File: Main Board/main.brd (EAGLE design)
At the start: 76.2 x 37.6 mm, 7 parts

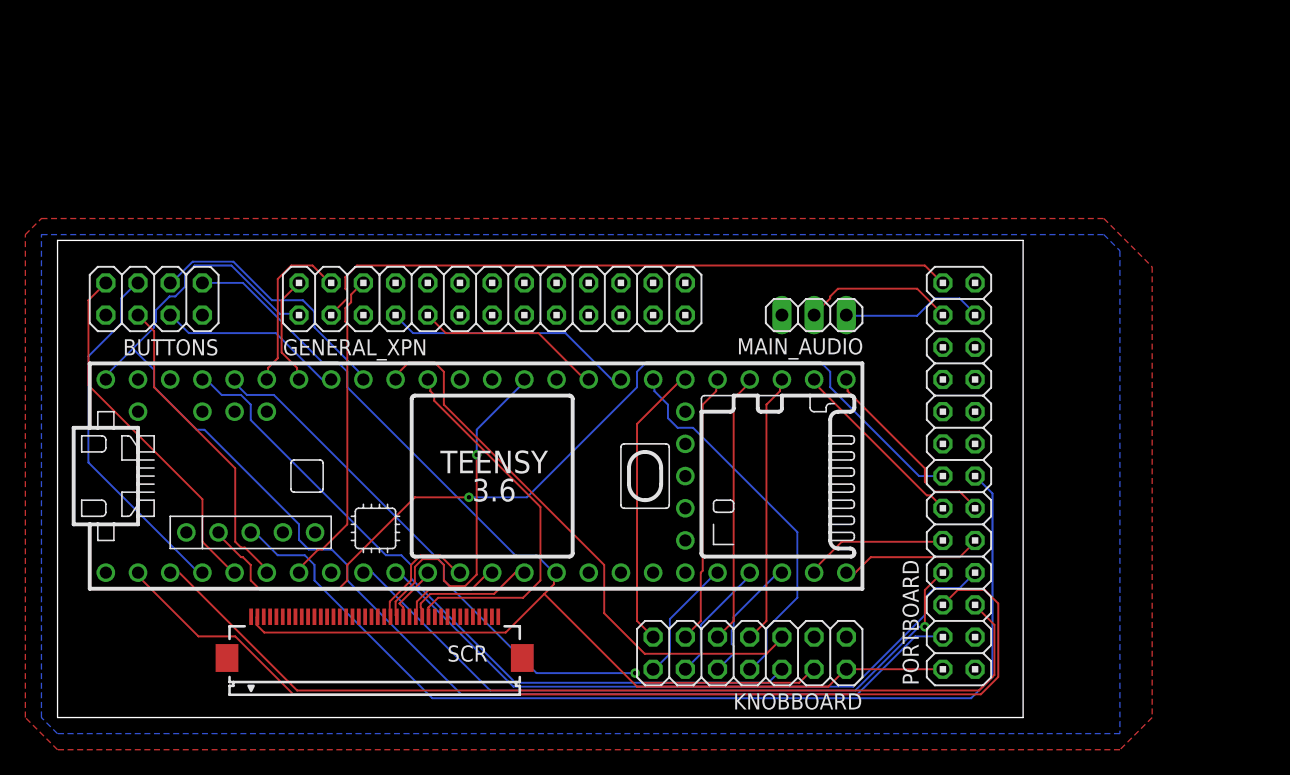
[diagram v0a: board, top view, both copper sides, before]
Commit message: Main Board Complete!
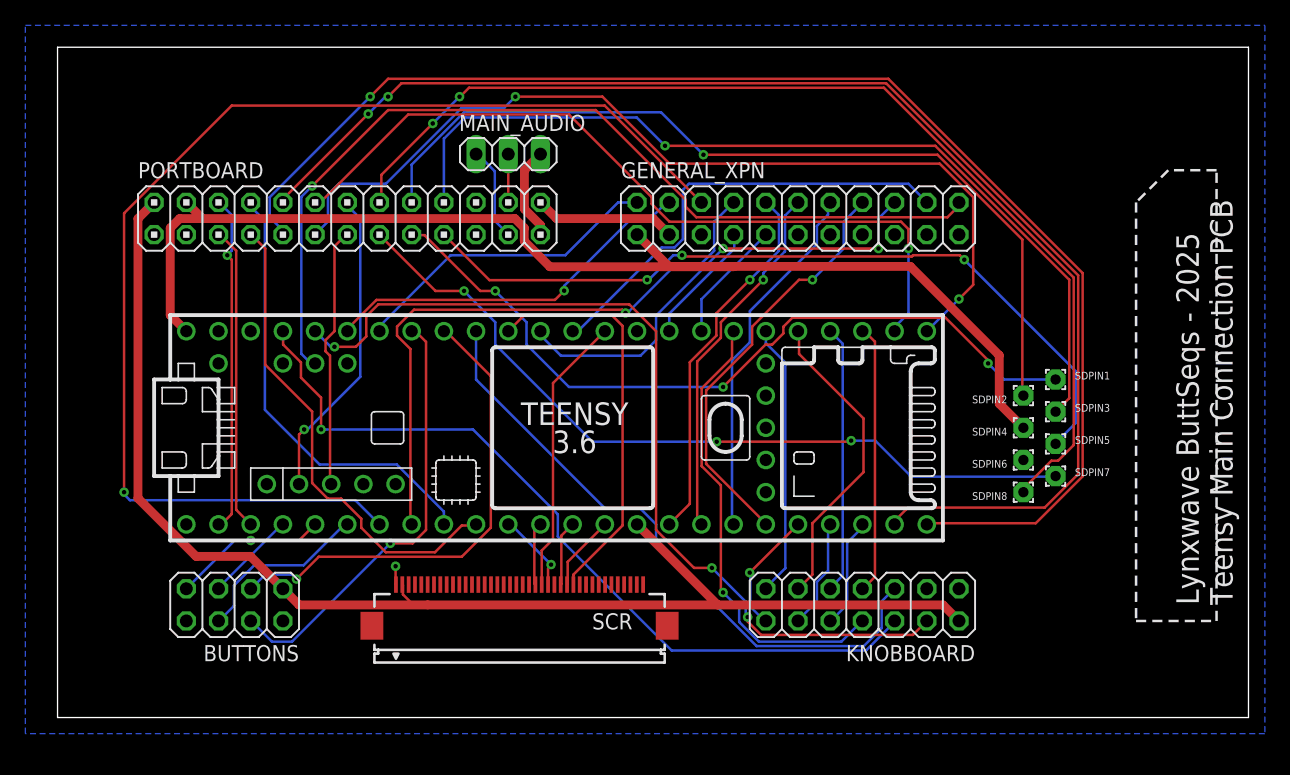
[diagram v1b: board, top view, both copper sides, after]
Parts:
- added SDPIN1, SDPIN2, SDPIN3, SDPIN4, SDPIN5, SDPIN6, SDPIN7, SDPIN8: (no value), wirepad:1,6/0,8
- GENERAL_XPN: device pinhead:2X13 -> pinhead:2X11
- moved PORTBOARD 52.4 mm to (22.9, 39.4), turned to 0 degrees
- moved MAIN_AUDIO 27.3 mm to (35.6, 44.5), turned to 0 degrees
- moved BUTTONS 25.0 mm to (14.0, 8.89)
- moved GENERAL_XPN 25.0 mm to (58.4, 39.4)
- moved SCR 11.7 mm to (36.4, 7.24)
- moved KNOBBOARD 9.67 mm to (63.5, 8.89)
- moved TEENSY_3.6 7.41 mm to (38.1, 22.9)
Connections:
- net AUDIO_L renamed OUTPUT_L
- net AUDIO_R renamed OUTPUT_R
- net SPI_CLK renamed XPN_CLK
- net SPI_MISO renamed XPN_MISO
- net SPI_MOSI renamed XPN_MOSI
- removed net AUDIO_0: GENERAL_XPN.11
- removed net AUDIO_1: GENERAL_XPN.13
- removed net AUDIO_2: GENERAL_XPN.15
- removed net AUDIO_3: GENERAL_XPN.17
- removed net AUDIO_4: GENERAL_XPN.19
- removed net AUDIO_5: GENERAL_XPN.21
- removed net AUDIO_6: GENERAL_XPN.23
- removed net AUDIO_7: GENERAL_XPN.25
- removed net N$10: TEENSY_3.6.25
- removed net N$11: TEENSY_3.6.26
- removed net N$12: TEENSY_3.6.27
- removed net N$25: TEENSY_3.6.15/A1
- removed net N$26: TEENSY_3.6.14/A0
- removed net N$6: TEENSY_3.6.6
- removed net N$9: TEENSY_3.6.24
- removed net SPI_CS: GENERAL_XPN.8
- removed net XPN_CV0: GENERAL_XPN.12
- removed net XPN_CV1: GENERAL_XPN.14
- removed net XPN_CV2: GENERAL_XPN.16
- removed net XPN_CV3: GENERAL_XPN.18
- removed net XPN_CV4: GENERAL_XPN.20
- removed net XPN_CV5: GENERAL_XPN.22
- removed net XPN_CV6: GENERAL_XPN.24
- removed net XPN_CV7: GENERAL_XPN.26
- new net XPN_CS0: GENERAL_XPN.8, TEENSY_3.6.6
- new net XPN_CS1: GENERAL_XPN.10, TEENSY_3.6.24
- new net XPN_CS2: GENERAL_XPN.12, TEENSY_3.6.25
- new net XPN_CS3: GENERAL_XPN.14, TEENSY_3.6.26
- new net XPN_CS4: GENERAL_XPN.16, TEENSY_3.6.27
- new net XPN_CS5: GENERAL_XPN.18, TEENSY_3.6.15/A1
- new net XPN_CS6: GENERAL_XPN.20, TEENSY_3.6.14/A0
- new net XPN_CS7: GENERAL_XPN.22, TEENSY_3.6.A10
- net +5V: now also SDPIN4.1
- net GND: now also SDPIN6.1
- net SDCLK: now also SDPIN5.1
- net SDCMD: now also SDPIN3.1
- net SDDATA0: now also SDPIN7.1
- net SDDATA1: now also SDPIN8.1
- net SDDATA2: now also SDPIN1.1
- net SDDATA3: now also SDPIN2.1
- net TEENSY_L: now also GENERAL_XPN.9; no longer GENERAL_XPN.7
- net TEENSY_R: now also GENERAL_XPN.7; no longer GENERAL_XPN.9
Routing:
- net MIDIOUT3: track 11.3 -> 107.6 mm, vias 0 -> 1
- net MIDIIN3: track 11.4 -> 105.1 mm, vias 0 -> 2
- net SDDATA1: track 0.00 -> 84.9 mm, vias 0 -> 2
- net XPN_CS7: track 0.00 -> 73.0 mm, vias 0 -> 1
- net SDCMD: track 0.00 -> 71.2 mm, vias 0 -> 1
- net XPN_MISO: track 25.3 -> 95.5 mm, vias 0 -> 1
- net SDDATA3: track 0.00 -> 69.4 mm, vias 0 -> 1
- net SDCLK: track 0.00 -> 62.7 mm, vias 0 -> 3
- net SDDATA0: track 0.00 -> 62.5 mm, vias 0 -> 3
- net SDDATA2: track 0.00 -> 61.5 mm, vias 0 -> 3
- net USBDATA+: track 81.8 -> 20.6 mm
- net MIDIOUT4: track 15.6 -> 73.0 mm, vias 0 -> 2
- net MIDIIN1: track 83.7 -> 26.7 mm, vias 0 -> 1
- net MIDIOUT1: track 75.5 -> 24.0 mm
- net XPN_CS0: track 0.00 -> 48.2 mm, vias 0 -> 1
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- added copper zone on layer 16, net GND
- removed copper zone on layer 16, net AGND
- removed copper zone on layer 1, net GND
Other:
- board size 76.2 x 37.6 mm -> 94 x 52.9 mm
- board text added: "Lynxwave ButtSeqs - 2025 Teensy Main Connection PCB"
